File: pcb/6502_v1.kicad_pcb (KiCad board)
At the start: 2 copper layers, 174.6 x 126.8 mm, 96 parts, among them J1 Jack-DC, J10 V_SLCT, J11 ACPort2, J12 WE_Cont, J2 Screw_Terminal_01x02, J3 VBus-80, J4 NMI_Contr, J5 JTAG, J6 KeyboardCon, J7 PORTA, J8 PORTB, J9 ACPort1, Q1 NMOS, Q2 NMOS, Q3 NMOS, Q4 NMOS, Q5 NMOS, Q6 NMOS, Q7 NMOS, Q8 NMOS, SW1 SW_Push, U1 74HC14, U10 L7805, U11 LD1117V33, U12 74HC595, U14 6522, U15 6502, U2 28C256, U3 CY62256-70PC, U5 6522, U6 W65C51NxP, U7 W65C51NxP, U8 EPM7128SLC84-15, U9 74AHC595, Y1 1.8432mHz, Y2 50mHz, Y3 Crystal

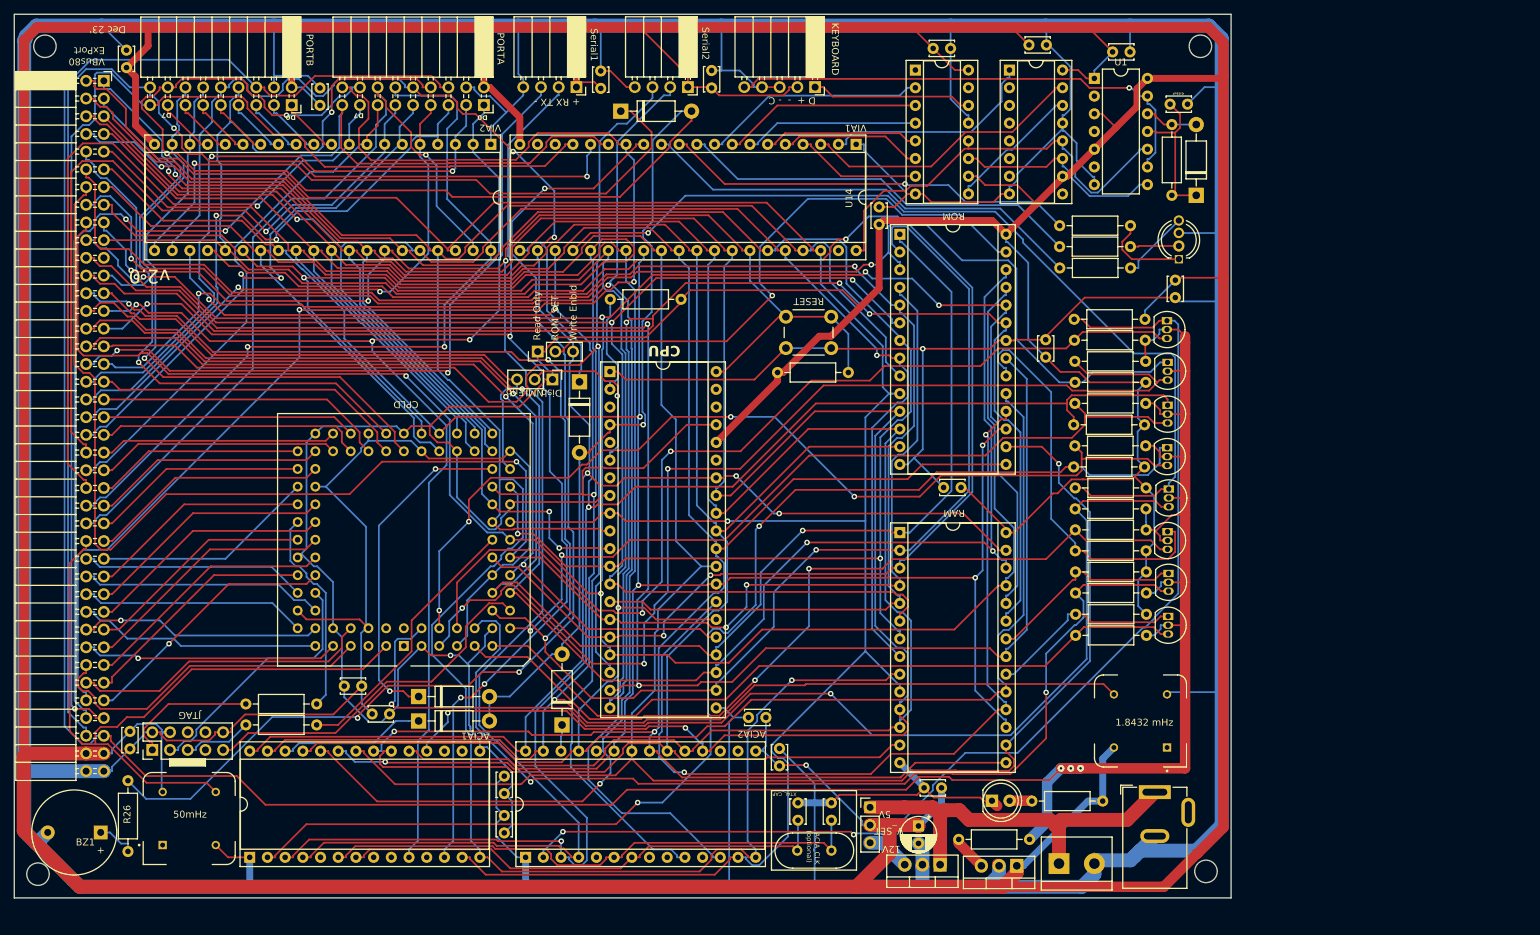
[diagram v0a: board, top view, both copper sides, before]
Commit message: V4 Pcb Upload.
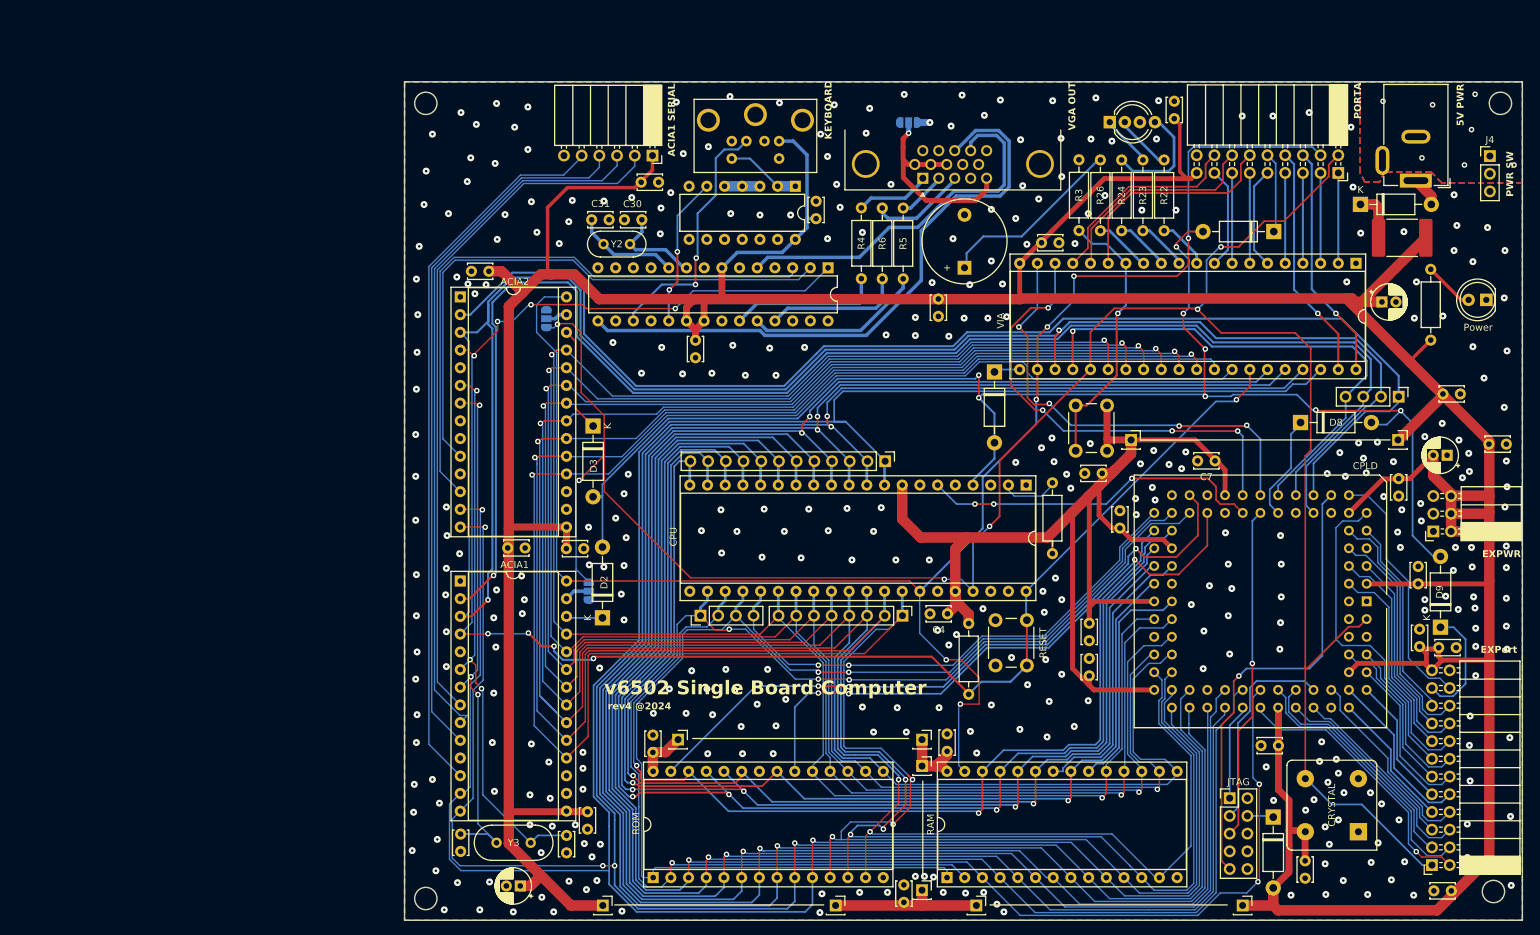
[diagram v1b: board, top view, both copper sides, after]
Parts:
- removed the C2 at (121.2, 125.5)
- removed C98, C99: 0.1uF, Capacitor_THT:C_Disc_D3.4mm_W2.1mm_P2.50mm
- removed D1: PWR_LED, LED_THT:LED_D5.0mm
- removed J11: ACPort2, Connector_PinSocket_2.54mm:PinSocket_1x04_P2.54mm_Horizontal
- removed Q1, Q2, Q3, Q4, Q5, Q6, Q7, Q8: NMOS, Package_TO_SOT_THT:TO-92_Inline
- removed R10, R11, R12, R16, R17, R18, R19, R20, R21, R7, R8, R9: 10k, Resistor_THT:R_Axial_DIN0207_L6.3mm_D2.5mm_P10.16mm_Horizontal
- removed R14: 1K, Resistor_THT:R_Axial_DIN0207_L6.3mm_D2.5mm_P10.16mm_Horizontal
- removed R15: 10K, Resistor_THT:R_Axial_DIN0207_L6.3mm_D2.5mm_P10.16mm_Horizontal
- removed R25: ?, Resistor_THT:R_Axial_DIN0207_L6.3mm_D2.5mm_P10.16mm_Horizontal
- removed R28: R, Resistor_THT:R_Axial_DIN0207_L6.3mm_D2.5mm_P10.16mm_Horizontal
- removed SW1: SW_Push, Button_Switch_THT:SW_PUSH_6mm_H4.3mm
- removed U10: L7805, Package_TO_SOT_THT:TO-220-3_Vertical
- removed U11: LD1117V33, Package_TO_SOT_THT:TO-220-3_Vertical
- removed U12: 74HC595, Package_DIP:DIP-16_W7.62mm_Socket
- removed U14: 6522, Package_DIP:DIP-40_W15.24mm_Socket
- removed U15: 6502, Package_DIP:DIP-40_W15.24mm_Socket
- removed U2: 28C256, Package_DIP:DIP-28_W15.24mm_Socket
- removed U3: CY62256-70PC, Package_DIP:DIP-28_W15.24mm_Socket
- removed U6: W65C51NxP, Package_DIP:DIP-28_W15.24mm_Socket
- removed U8: EPM7128SLC84-15, Package_LCC:PLCC-84_THT-Socket
- removed U9: 74AHC595, Package_DIP:DIP-16_W7.62mm_Socket
- removed Y1: 1.8432mHz, crystal:OSC_ECS-2100AX-200
- added ACIA1: W65C51NxP, Package_DIP:DIP-28_W15.24mm_Socket, F.Cu at (77.4, 105.9)
- added C2: 0.01uF, Capacitor_THT:C_Disc_D3.4mm_W2.1mm_P2.50mm, F.Cu at (217.8, 115.5)
- added C2: 0.01uF, Capacitor_THT:C_Disc_D3.4mm_W2.1mm_P2.50mm, F.Cu at (111.2, 71.4)
- added C20: 0.01uF, Capacitor_THT:C_Disc_D3.4mm_W2.1mm_P2.50mm, F.Cu at (198.6, 146.1)
- added C21: 0.01uF, Capacitor_THT:C_Disc_D3.4mm_W2.1mm_P2.50mm, F.Cu at (141.1, 152.0)
- added C22: 0.01uF, Capacitor_THT:C_Disc_D3.4mm_W2.1mm_P2.50mm, F.Cu at (103.3, 48.7)
- added C23: 0.01uF, Capacitor_THT:C_Disc_D3.4mm_W2.1mm_P2.50mm, F.Cu at (225.0, 86.3)
- added C27: 0.01uF, Capacitor_THT:C_Disc_D3.4mm_W2.1mm_P2.50mm, F.Cu at (214.9, 106.3)
- added C28: 0.01uF, Capacitor_THT:C_Disc_D3.4mm_W2.1mm_P2.50mm, F.Cu at (212.1, 91.2)
- added C29: 0.01uF, Capacitor_THT:C_Disc_D3.4mm_W2.1mm_P2.50mm, F.Cu at (169.5, 90.5)
- added C30: C, Capacitor_THT:C_Disc_D3.4mm_W2.1mm_P2.50mm, F.Cu at (103.5, 54.1)
- added C31: C, Capacitor_THT:C_Disc_D3.4mm_W2.1mm_P2.50mm, F.Cu at (96.3, 54.1)
- added C32: MainC, Capacitor_THT:CP_Radial_D5.0mm_P2.00mm, F.Cu at (86.0, 149.7)
- added C33: C, Capacitor_THT:CP_Radial_D5.0mm_P2.00mm, F.Cu at (209.7, 65.9)
- added C34: C, Capacitor_THT:CP_Radial_D5.0mm_P2.00mm, F.Cu at (219.0, 87.9)
- added C9: 0.01uF, Capacitor_THT:C_Disc_D3.4mm_W2.1mm_P2.50mm, F.Cu at (81.5, 61.5)
- added CPLD: EPM7128SLC84-15, Package_LCC:PLCC-84_THT-Socket, F.Cu at (207.5, 108.8)
- added CPU: 6502, Package_DIP:DIP-40_W15.24mm_Socket, F.Cu at (158.6, 92.2)
- added CRYSTAL: 1.8432mHz, Oscillator:Oscillator_DIP-8_LargePads, F.Cu at (206.3, 141.9)
- added D11: 1N4001, Diode_THT:D_DO-41_SOD81_P10.16mm_Horizontal, F.Cu at (194.1, 139.8)
- added D9: SB140, Diode_THT:D_DO-41_SOD81_P10.16mm_Horizontal, F.Cu at (218.1, 112.6)
- added F1: Fuse, Fuse:Fuse_2920_7451Metric, F.Cu at (212.6, 56.7)
- added J13: Debug_ADR1, Connector_PinHeader_2.54mm:PinHeader_1x04_P2.54mm_Vertical, F.Cu at (111.9, 110.9)
- added J14: VGA_Conf, Jumper:SolderJumper-3_P1.3mm_Open_RoundedPad1.0x1.5mm_NumberLabels, B.Cu at (141.7, 40.1)
- added J15: PW_JMP, Connector_PinSocket_2.54mm:PinSocket_1x01_P2.54mm_Vertical, F.Cu at (212.0, 85.7)
- added J16: EN, Jumper:SolderJumper-3_P1.3mm_Open_RoundedPad1.0x1.5mm_NumberLabels, B.Cu at (95.9, 107.4)
- added J17: PW_JMP, Connector_PinSocket_2.54mm:PinSocket_1x01_P2.54mm_Vertical, F.Cu at (143.7, 132.5)
- added J18: PW_JMP, Connector_PinSocket_2.54mm:PinSocket_1x01_P2.54mm_Vertical, F.Cu at (131.3, 152.5)
- added J19: PW_JMP, Connector_PinSocket_2.54mm:PinSocket_1x01_P2.54mm_Vertical, F.Cu at (189.7, 152.5)
- added J20: PW_JMP, Connector_PinSocket_2.54mm:PinSocket_1x01_P2.54mm_Vertical, F.Cu at (143.7, 150.3)
- added J21: PW_JMP, Connector_PinSocket_2.54mm:PinSocket_1x01_P2.54mm_Vertical, F.Cu at (97.9, 152.5)
- added J22: PW_JMP, Connector_PinSocket_2.54mm:PinSocket_1x01_P2.54mm_Vertical, F.Cu at (173.7, 85.7)
- added J23: PW_JMP, Connector_PinSocket_2.54mm:PinSocket_1x01_P2.54mm_Vertical, F.Cu at (108.7, 128.7)
- added J24: PW_JMP, Connector_PinSocket_2.54mm:PinSocket_1x01_P2.54mm_Vertical, F.Cu at (151.5, 152.5)
- added J26: ACIAPort, Connector_PinSocket_2.54mm:PinSocket_1x06_P2.54mm_Horizontal, F.Cu at (105.0, 44.9)
- added J28: PW_JMP, Connector_PinSocket_2.54mm:PinSocket_1x01_P2.54mm_Vertical, F.Cu at (143.7, 128.7)
- added JTAG: JTAG, Connector_PinHeader_2.54mm:PinHeader_2x05_P2.54mm_Vertical, F.Cu at (187.8, 137.1)
- added Power: PWR_LED, LED_THT:LED_D5.0mm, F.Cu at (224.6, 65.6)
- added RAM: CY62256-70PC, Package_DIP:DIP-28_W15.24mm_Socket, F.Cu at (147.2, 148.5)
- added RESET: RESET, Button_Switch_THT:SW_PUSH_6mm_H4.3mm, F.Cu at (158.7, 111.5)
- added ROM: 28C256, Package_DIP:DIP-28_W15.24mm_Socket, F.Cu at (105.1, 148.5)
- added SW2: SW_Push, Button_Switch_THT:SW_PUSH_6mm_H4.3mm, F.Cu at (165.7, 87.2)
- added U4: 74HC00, Package_DIP:DIP-14_W7.62mm, F.Cu at (125.5, 49.3)
- C1, C10, C11, C12, C13, C15, C16, C17, C19, C24, C25, C26, C3, C4, C5, C6, C7, C8: value 0.1uF -> 0.01uF
- C14: value 0.1uF -> 0.01uF; footprint Capacitor_THT:CP_Radial_D5.0mm_P2.50mm -> Capacitor_THT:C_Disc_D3.4mm_W2.1mm_P2.50mm
- D6: value SB140 -> D
- D8: value 1N4001 -> SB140
- J1: value Jack-DC -> VGA_Out; footprint Connector_BarrelJack:BarrelJack_GCT_DCJ200-10-A_Horizontal -> Connector_Dsub:DSUB-15-HD_Female_Horizontal_P2.29x1.98mm_EdgePinOffset3.03mm_Housed_MountingHolesOffset4.94mm
- J10: value V_SLCT -> PS2-MINIDIN6-FEMALE; footprint Connector_PinHeader_2.54mm:PinHeader_1x03_P2.54mm_Vertical -> kicad_sym:MINI-DIN-6-FULL-SHIELD
- J12: value WE_Cont -> Debug_CS; footprint Connector_PinHeader_2.54mm:PinHeader_1x03_P2.54mm_Vertical -> Connector_PinHeader_2.54mm:PinHeader_1x04_P2.54mm_Vertical
- J2: value Screw_Terminal_01x02 -> DC; footprint TerminalBlock:TerminalBlock_bornier-2_P5.08mm -> Connector_BarrelJack:BarrelJack_GCT_DCJ200-10-A_Horizontal
- J3: value VBus-80 -> Debug_DATA; footprint Connector_PinSocket_2.54mm:PinSocket_2x40_P2.54mm_Horizontal -> Connector_PinHeader_2.54mm:PinHeader_1x08_P2.54mm_Vertical
- J4: value NMI_Contr -> PWR-SW
- J5: value JTAG -> Debug_ADR0; footprint Connector_PinHeader_2.54mm:PinHeader_2x05_P2.54mm_Vertical -> Connector_PinHeader_2.54mm:PinHeader_1x12_P2.54mm_Vertical
- J6: value KeyboardCon -> EN; footprint Connector_PinSocket_2.54mm:PinSocket_1x05_P2.54mm_Horizontal -> Jumper:SolderJumper-3_P1.3mm_Open_RoundedPad1.0x1.5mm_NumberLabels; moved to B.Cu
- J8: value PORTB -> ExpandBus; footprint Connector_PinSocket_2.54mm:PinSocket_2x09_P2.54mm_Horizontal -> Connector_PinSocket_2.54mm:PinSocket_2x12_P2.54mm_Horizontal
- J9: value ACPort1 -> ExpandPower; footprint Connector_PinSocket_2.54mm:PinSocket_1x04_P2.54mm_Horizontal -> Connector_PinSocket_2.54mm:PinSocket_2x03_P2.54mm_Horizontal
- R3, R4, R5, R6: value 10k -> 1K
- U1: value 74HC14 -> ATmega328-P; footprint Package_DIP:DIP-14_W7.62mm -> Package_DIP:DIP-28_W7.62mm
- Y2: value 50mHz -> Crystal; footprint crystal:OSC_ECS-2100AX-200 -> Crystal:Crystal_HC52-U_Vertical
- moved J8 196.6 mm to (216.8, 146.7), turned to 180 degrees
- moved R26 160.3 mm to (169.2, 55.7), turned to 90 degrees
- moved D6 152.5 mm to (206.6, 51.9)
- moved C6 148.4 mm to (160.8, 57.4), turned to 0 degrees
- moved BZ1 148.1 mm to (149.8, 61.0), turned to 90 degrees
- moved J9 138.5 mm to (217.0, 98.8), turned to 180 degrees
- moved J4 138.3 mm to (225.1, 44.9), turned to 0 degrees
- moved J3 137.9 mm to (140.8, 110.9), turned to -90 degrees
- moved C10 137.4 mm to (167.7, 119.5)
- moved C7 129.1 mm to (185.7, 88.7), turned to 180 degrees
- moved C15 125.6 mm to (95.7, 139.0), turned to -90 degrees
- moved U5 125.3 mm to (205.9, 60.3)
- moved D5 124.3 mm to (194.1, 55.8), turned to 180 degrees
- moved J12 123.7 mm to (212.1, 79.5), turned to -90 degrees
- moved J7 123.0 mm to (203.4, 47.4)
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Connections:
- C17 pad 1: VCC -> ACIAXT1
- C18 pad 1: GND -> VCC
- C18 pad 2: Net-(D8-K) -> GND
- C19 pad 1: VCC -> ACIAXT2
- C25 pad 1: GND -> VCC
- C25 pad 2: VCC -> GND
- C26 pad 1: GND -> VCC
- C26 pad 2: VCC -> GND
- D6 pad 2: IRQ -> Net-(D6-A)
- D8 pad 2: Net-(D8-A) -> IRQ
- J1 pad 1: Net-(J10-Pin_1) -> VGA_R
- J1 pad 2: GND -> VGA_G
- J1 pad 3: (no net) -> VGA_B
- J10 pad 1: Net-(J10-Pin_1) -> KEYB_DATA
- J10 pad 2: VCC -> unconnected-(J10-DATA2/NC-Pad2)
- J10 pad 3: Net-(J10-Pin_3) -> GND
- J12 pad 1: VCC -> ACIA2CS1
- J12 pad 2: Net-(J12-Pin_2) -> IACSB
- J12 pad 3: RWB -> ACIA1CS1
- J2 pad 1: Net-(J10-Pin_1) -> Net-(D6-A)
- J2 pad 2: GND -> Net-(J4-Pin_2)
- J3 pad 2: A0 -> D1
- J3 pad 3: D1 -> D2
- J3 pad 4: A1 -> D3
- J3 pad 5: D2 -> D4
- J3 pad 6: A2 -> D5
- J3 pad 7: D3 -> D6
- J3 pad 8: A3 -> D7
- J4 pad 1: VCC -> unconnected-(J4-Pin_1-Pad1)
- J4 pad 2: NMIC -> Net-(J4-Pin_2)
- J4 pad 3: NMIB -> GND
- J5 pad 1: Net-(J5-Pin_1) -> A0
- J5 pad 10: GND -> A9
- J5 pad 2: GND -> A1
- J5 pad 3: TDO -> A2
- J5 pad 4: VCC -> A3
- J5 pad 5: Net-(J5-Pin_5) -> A4
- J5 pad 6: unconnected-(J5-Pin_6-Pad6) -> A5
- J5 pad 7: unconnected-(J5-Pin_7-Pad7) -> A6
- J5 pad 8: unconnected-(J5-Pin_8-Pad8) -> A7
- J5 pad 9: TDI -> A8
- J6 pad 1: KEYB_DATA -> CLK
- J6 pad 2: VCC -> Net-(J6-Pin_2)
- J6 pad 3: GND -> (no net)
- J7 pad 1: PORTAD0 -> PORTA0
- J7 pad 10: RWB -> Net-(D5-K)
- J7 pad 11: PORTAD5 -> PORTA5
- J7 pad 12: CA1 -> SYS_CONT_D6
- J7 pad 13: PORTAD6 -> PORTA6
- J7 pad 14: CA2 -> SYS_CONT_D7
- J7 pad 15: PORTAD7 -> PORTA7
- J7 pad 16: IRQ -> SYS_CONT_D8
- J7 pad 17: SYS_CONT_D6 -> VCC
- J7 pad 18: SYS_CONT_D5 -> GND
- J7 pad 2: VCC -> CLK
- J7 pad 3: PORTAD1 -> PORTA1
- J7 pad 4: GND -> RWB
- J7 pad 5: PORTAD2 -> PORTA2
- J7 pad 6: +3V0 -> CA1
- J7 pad 7: PORTAD3 -> PORTA3
- J7 pad 8: CLK -> CA2
- J7 pad 9: PORTAD4 -> PORTA4
- J8 pad 1: PORTBD0 -> CLK
- J8 pad 10: RWB -> EBB5
- J8 pad 11: PORTBD5 -> EBA4
- J8 pad 12: CB1 -> EBB4
- J8 pad 13: PORTBD6 -> EBA3
- J8 pad 14: CB2 -> EBB3
- J8 pad 15: PORTBD7 -> EBA2
- J8 pad 16: IRQ -> EBB2
- J8 pad 17: SYS_CONT_D8 -> EBA1
- J8 pad 18: SYS_CONT_D7 -> EBB1
- J8 pad 2: VCC -> CPRES
- J8 pad 3: PORTBD1 -> EBC0
- J8 pad 4: GND -> EBC2
- J8 pad 5: PORTBD2 -> EBA7
- J8 pad 6: +3V0 -> EBB7
- J8 pad 7: PORTBD3 -> EBA6
- J8 pad 8: CLK -> EBB6
- J8 pad 9: PORTBD4 -> EBA5
- J9 pad 1: VCC -> GND
- J9 pad 2: ACIA1RX -> VCC
- J9 pad 3: ACIA1TX -> GND
- J9 pad 4: GND -> VCC
- R3 pad 1: IO4 -> SYS_CONT_D5
- R3 pad 2: +3V0 -> GND
- R4 pad 1: VCC -> Net-(U1-PC0)
- R4 pad 2: ACIA1CS1 -> VGA_R
- R5 pad 1: VCC -> Net-(U1-PC1)
- R5 pad 2: ACIA2CS1 -> VGA_G
- R6 pad 1: IO5 -> Net-(U1-PC2)
- R6 pad 2: +3V0 -> VGA_B
- U1 pad 1: VCC -> RESB
- U1 pad 10: VIA1CA1 -> Net-(U1-XTAL2/PB7)
- U1 pad 11: Net-(D8-K) -> unconnected-(U1-PD5-Pad11)
- U1 pad 12: Net-(D8-A) -> unconnected-(U1-PD6-Pad12)
- U1 pad 13: KEYB_CLK -> unconnected-(U1-PD7-Pad13)
- U1 pad 14: VCC -> unconnected-(U1-PB0-Pad14)
- U1 pad 2: unconnected-(U1-Pad2) -> ACIA2TX
- U1 pad 3: VCC -> ACIA2RX
- U1 pad 5: VCC -> VSync
- U1 pad 7: GND -> VCC
- U1 pad 8: Net-(U12-SRCLK) -> GND
- U1 pad 9: KEYB_CLK -> Net-(U1-XTAL1/PB6)
- U5 pad 10: PORTBD0 -> SYS_CONT_D1
- U5 pad 11: PORTBD1 -> SYS_CONT_D2
- U5 pad 12: PORTBD2 -> SYS_CONT_D3
- U5 pad 13: PORTBD3 -> SYS_CONT_D4
- U5 pad 14: PORTBD4 -> SYS_CONT_D5
- U5 pad 15: PORTBD5 -> SYS_CONT_D6
- U5 pad 16: PORTBD6 -> SYS_CONT_D7
- U5 pad 17: PORTBD7 -> SYS_CONT_D8
- U5 pad 2: PORTAD0 -> PORTA0
- U5 pad 21: Net-(D3-K) -> Net-(D4-K)
- U5 pad 24: VIA2CS1 -> VIACS1
- U5 pad 3: PORTAD1 -> PORTA1
- U5 pad 4: PORTAD2 -> PORTA2
- U5 pad 5: PORTAD3 -> PORTA3
- U5 pad 6: PORTAD4 -> PORTA4
- U5 pad 7: PORTAD5 -> PORTA5
- U5 pad 8: PORTAD6 -> PORTA6
- U5 pad 9: PORTAD7 -> PORTA7
- U7 pad 26: Net-(D5-K) -> Net-(D3-K)
- U7 pad 27: CLK -> Net-(J6-Pin_2)
- U7 pad 6: Net-(U6-XTAL1) -> ACIAXT1
- U7 pad 7: Net-(U6-XTAL2) -> ACIAXT2
- U7 pad 8: unconnected-(U7-~{RTS}-Pad8) -> ACIA2RTS
- U7 pad 9: unconnected-(U7-~{CTS}-Pad9) -> ACIA2CTS
- Y2 pad 1: (no net) -> Net-(U1-XTAL2/PB7)
- Y3 pad 1: Net-(U6-XTAL2) -> ACIAXT2
- Y3 pad 2: Net-(U6-XTAL1) -> ACIAXT1
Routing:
- net GND: track 1197.1 -> 1.75 mm, vias 1 -> 363
- net +3V0: track 453.1 -> 0.00 mm, vias 3 -> 0
- net VCC: track 1293.5 -> 886.4 mm, vias 2 -> 0
- net VIA2CS1: track 162.9 -> 0.00 mm, vias 1 -> 0
- net IO2: track 160.2 -> 0.00 mm, vias 2 -> 0
- net IO3: track 159.2 -> 0.00 mm, vias 3 -> 0
- net SYS_CONT_D5: track 195.8 -> 39.5 mm, vias 2 -> 1
- net SYS_CONT_D7: track 183.7 -> 31.1 mm, vias 2 -> 0
- net SYS_CONT_D4: track 160.3 -> 8.13 mm, vias 3 -> 0
- net IO7: track 146.5 -> 0.00 mm, vias 2 -> 0
- net SYS_CONT_D8: track 176.1 -> 29.6 mm, vias 1 -> 0
- net IO5: track 142.4 -> 0.00 mm, vias 2 -> 0
- net SYS_CONT_D6: track 169.8 -> 32.1 mm, vias 2 -> 0
- net IO4: track 136.0 -> 0.00 mm, vias 4 -> 0
- net VIA1CS1: track 133.1 -> 0.00 mm, vias 1 -> 0
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- added copper zone on B.Cu, net GND
- added copper zone on F.Cu, net GND
- added copper zone on B.Cu, net Net-(J4-Pin_2)
- added copper zone on F.Cu, net Net-(J4-Pin_2)
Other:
- board size 174.6 x 126.8 mm -> 160.4 x 120.3 mm
- board text added: "5V PWR"
- board text added: "ACIA1 SERIAL"
- board text added: "EXPWR"
- board text added: "EXPort"
- board text added: "PWR SW"
- board text added: "VGA OUT"
- board text added: "VIA"
- board text added: "rev4 @2024"
- board text added: "v6502 Single Board Computer"
- board text removed: "+ RX TX -"
- board text removed: "0.01uF"
- board text removed: "1.8432 mHz"
- board text removed: "12V"
- board text removed: "50mHz"
- board text removed: "5V"
- board text removed: "ACIA1"
- board text removed: "ACIA_CLK (optional)"
- board text removed: "CPLD"
- board text removed: "CPU"
- board text removed: "D + - - C"
- board text removed: "D0"
- board text removed: "D7"
- board text removed: "Dec 23'"
- board text removed: "December 2023 - Vatan Zengin"
- board text removed: "Disb"
- board text removed: "Enb"
- board text removed: "JTAG"
- board text removed: "NMI"
- board text removed: "PORTB"
- board text removed: "PWR"
- board text removed: "RAM"
- board text removed: "RESET"
- board text removed: "ROM"
- board text removed: "ROM_SET"
- board text removed: "Read Only"
- board text removed: "Refer the documentation for hardware configurations."
- board text removed: "SRAM"
- board text removed: "Serial1"
- board text removed: "Serial2"
- board text removed: "VBus80 ExPort"
- board text removed: "VIA1"
- board text removed: "VIA2"
- board text removed: "V_SET"
- board text removed: "Vatan's 6502 Single Board Computer v2"
- board text removed: "Write Enbld"
- board text removed: "XTAL_CAP"
- board text removed: "v2.0"
